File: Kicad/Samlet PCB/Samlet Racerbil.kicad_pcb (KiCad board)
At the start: 2 copper layers, 11 parts, among them J1 Pickit Forbindelse, J2 LED, J5 Conn_01x05_Female, Q1 IRL1404, U1 L7805, U2 PIC16F684-IP

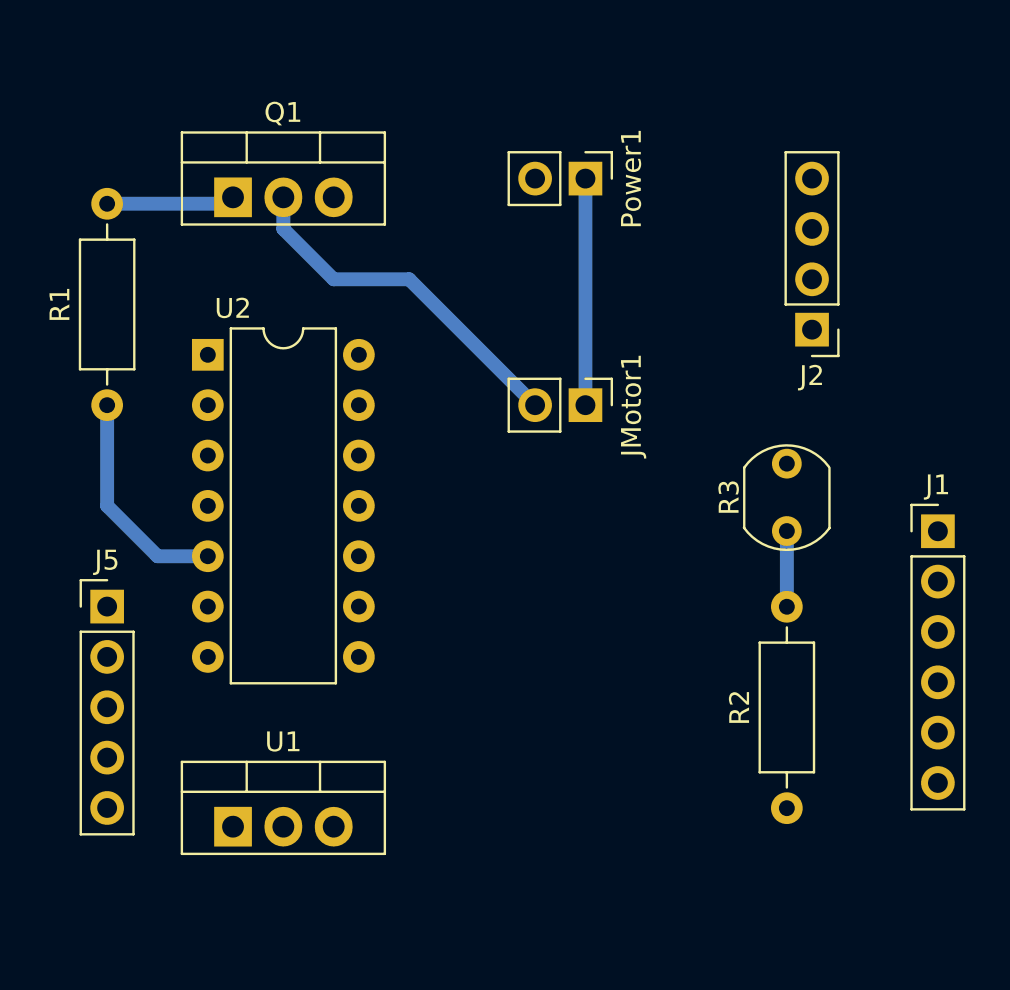
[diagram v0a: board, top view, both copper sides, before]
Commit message: update
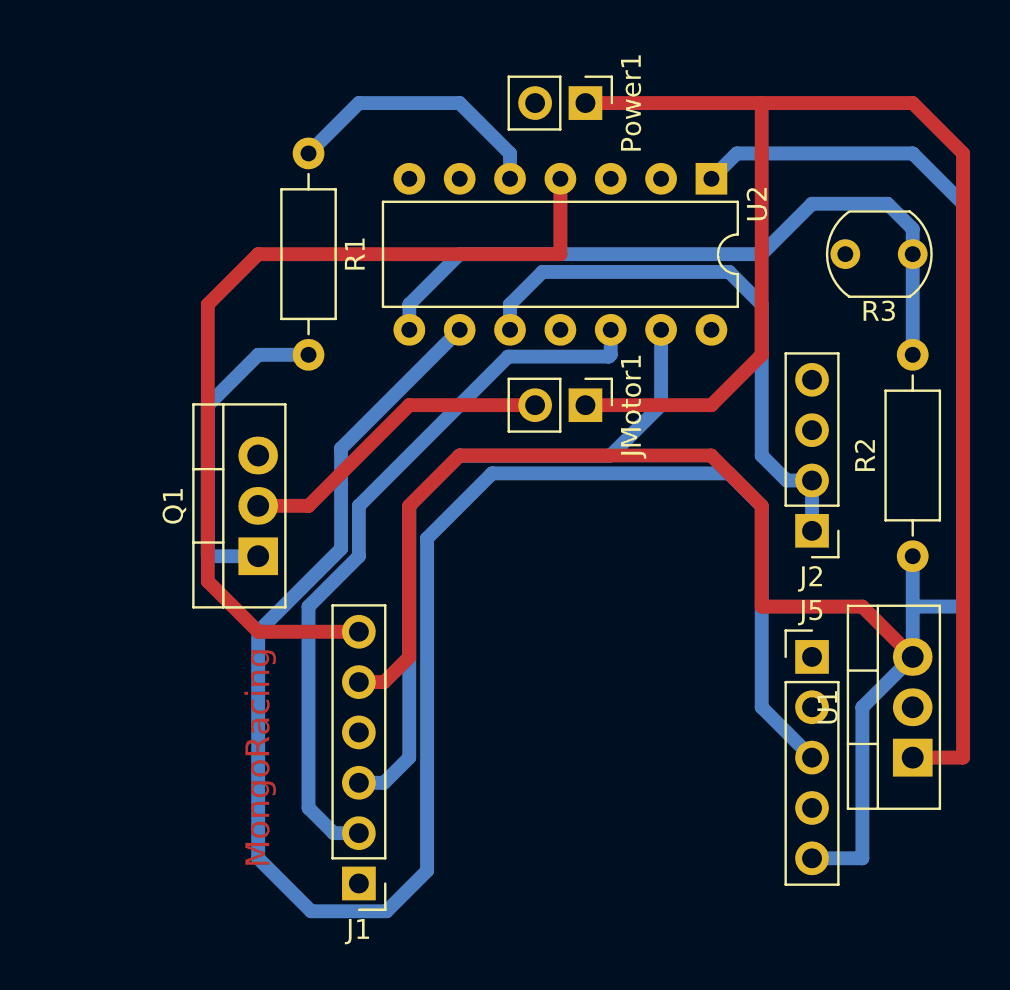
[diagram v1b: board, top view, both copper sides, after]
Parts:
- moved J5 35.7 mm to (147.3, 88.9)
- moved U1 34.5 mm to (152.4, 94.0), turned to 90 degrees
- moved J1 34.2 mm to (124.5, 100.3), turned to 180 degrees
- moved U2 26.9 mm to (142.2, 64.8), turned to -90 degrees
- moved Q1 18.1 mm to (119.4, 83.8), turned to 90 degrees
- moved R1 16.3 mm to (121.9, 63.5), turned to -90 degrees
- moved R3 15.3 mm to (152.4, 68.6), turned to 180 degrees
- moved R2 14.2 mm to (152.4, 83.8)
- moved J2 10.2 mm to (147.3, 82.5)
- moved Power1 3.81 mm to (135.9, 61.0)
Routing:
- net 5V: track 0.00 -> 100.3 mm
- net ACC: track 0.00 -> 90.8 mm
- net 12V: track 11.4 -> 75.8 mm
- net Net-(J1-Pad6): track 0.00 -> 45.3 mm
- net Net-(J1-Pad2): track 0.00 -> 36.5 mm
- net Net-(J1-Pad3): track 0.00 -> 34.4 mm
- net LDR: track 3.82 -> 35.7 mm
- net Lys: track 0.00 -> 28.6 mm
- net Net-(Q1-Pad1): track 6.48 -> 16.3 mm
- net PWM: track 11.2 -> 13.5 mm
- net Net-(JMotor1-Pad2): track 18.0 -> 16.1 mm
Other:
- board text added: "MongoRacing"
